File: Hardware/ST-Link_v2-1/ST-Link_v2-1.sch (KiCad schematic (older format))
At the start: 40 parts, among them J1 Conn_01x06, J2 USB_C_Receptacle, U1 STM32F103CBTx, U2 LP5907MFX-3.3, Y1 8Mhz

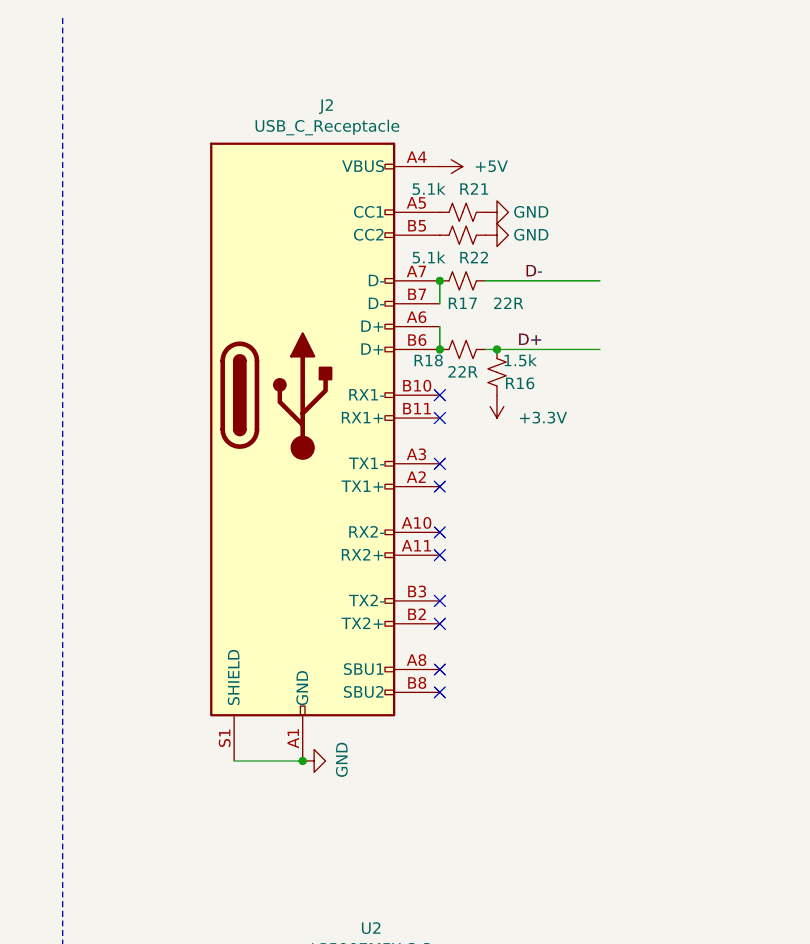
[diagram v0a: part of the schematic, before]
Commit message: V2.1 11/12/2021
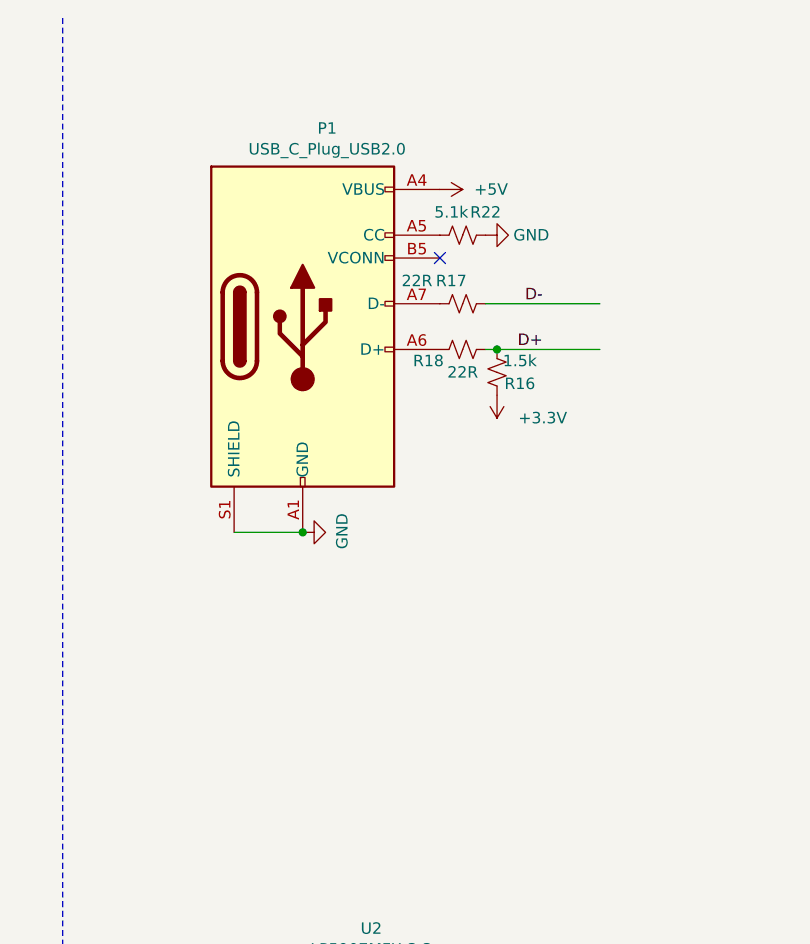
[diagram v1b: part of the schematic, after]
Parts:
- removed J2: USB_C_Receptacle, HKUST_RT_CONN:USB_C_MALE, symbol HKUST_RT_CONN:USB_C_Receptacle
- removed R21: 5.1k, HKUST_RT_RCL:R_0805_2012Metric, symbol HKUST_RT_RCL:R_Small_US
- added P1: USB_C_Plug_USB2.0, HKUST_RT_CONN:USB_C_MALE, symbol HKUST_RT_CONN:USB_C_Plug_USB2.0
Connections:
- wire segments 72 -> 70
- no-connect marks 28 -> 19
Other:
- moved on the sheet: R17
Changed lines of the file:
@@
 L HKUST_RT_RCL:R_Small_US R17
 U 1 1 619A5D6F
-P 6350 1650
-F 0 "R17" V 6450 1650 50  0000 C CNN
-F 1 "22R" V 6450 1850 50  0000 C CNN
-F 2 "HKUST_RT_RCL:R_0805_2012Metric" H 6418 1559 50  0001 L CNN
-F 3 "" H 6350 1650 50  0001 C CNN
-	1    6350 1650
+P 6350 1750
+F 0 "R17" V 6250 1700 50  0000 C CNN
+F 1 "22R" V 6250 1550 50  0000 C CNN
+F 2 "HKUST_RT_RCL:R_0805_2012Metric" H 6418 1659 50  0001 L CNN
+F 3 "" H 6350 1750 50  0001 C CNN
+	1    6350 1750
 	0    1    1    0
 $EndComp
@@
 Wire Notes Line style solid rgb(0, 0, 0)
 	4600 500  4600 7750
-Text Label 6700 1650 2    50   ~ 0
+Text Label 6700 1750 2    50   ~ 0
 D-
 Text Label 6700 1950 2    50   ~ 0
@@
 $EndComp
 $Comp
-L power:GND #PWR0102
-U 1 1 619EB02D
-P 5650 3750
-F 0 "#PWR0102" H 5650 3500 50  0001 C CNN
-F 1 "GND" H 5655 3577 50  0000 C CNN
-F 2 "" H 5650 3750 50  0001 C CNN
-F 3 "" H 5650 3750 50  0001 C CNN
-	1    5650 3750
-	0    -1   -1   0
-$EndComp
-$Comp
-L power:+5V #PWR0103
-U 1 1 619F8999
-P 6250 1150
-F 0 "#PWR0103" H 6250 1000 50  0001 C CNN
-F 1 "+5V" V 6250 1300 50  0000 L CNN
-F 2 "" H 6250 1150 50  0001 C CNN
-F 3 "" H 6250 1150 50  0001 C CNN
-	1    6250 1150
-	0    1    1    0
-$EndComp
-$Comp
-L HKUST_RT_RCL:R_Small_US R21
-U 1 1 61A837A5
-P 6350 1350
-F 0 "R21" V 6450 1300 50  0000 C CNN
-F 1 "5.1k" V 6450 1500 50  0000 C CNN
-F 2 "HKUST_RT_RCL:R_0805_2012Metric" H 6418 1259 50  0001 L CNN
-F 3 "" H 6350 1350 50  0001 C CNN
-	1    6350 1350
-	0    -1   -1   0
-$EndComp
-$Comp
 L power:GND #PWR0104
 U 1 1 61AA0D72
@@
 $EndComp
 Wire Wire Line
-	6950 1650 6450 1650
+	6950 1750 6450 1750
 $Comp
 L HKUST_RT_RCL:Crystal_GND24_Small Y1
@@
 	-1   0    0    1
 $EndComp
-Wire Wire Line
-	5350 3750 5650 3750
-NoConn ~ 6250 3050
-NoConn ~ 6250 2750
-NoConn ~ 6250 2850
-NoConn ~ 6250 3350
-NoConn ~ 6250 3450
-NoConn ~ 6250 2450
-NoConn ~ 6250 2550
-NoConn ~ 6250 2150
-Connection ~ 5650 3750
-$Comp
-L HKUST_RT_CONN:USB_C_Receptacle J2
-U 1 1 61AC3D44
-P 5650 2150
-F 0 "J2" H 5757 3417 50  0000 C CNN
-F 1 "USB_C_Receptacle" H 5757 3326 50  0000 C CNN
-F 2 "HKUST_RT_CONN:USB_C_MALE" H 5800 2150 50  0001 C CNN
-F 3 "https://www.usb.org/sites/default/files/documents/usb_type-c.zip" H 5800 2150 50  0001 C CNN
-	1    5650 2150
-	1    0    0    -1
-$EndComp
-NoConn ~ 6250 2250
-Wire Wire Line
-	6250 1650 6250 1750
-Wire Wire Line
-	6250 1850 6250 1950
+NoConn ~ 6250 1550
 $Comp
 L HKUST_RT_RCL:R_Small_US R22
 U 1 1 61AF811F
 P 6350 1450
-F 0 "R22" V 6250 1400 50  0000 C CNN
-F 1 "5.1k" V 6250 1600 50  0000 C CNN
+F 0 "R22" V 6450 1350 50  0000 C CNN
+F 1 "5.1k" V 6450 1500 50  0000 C CNN
 F 2 "HKUST_RT_RCL:R_0805_2012Metric" H 6418 1359 50  0001 L CNN
 F 3 "" H 6350 1450 50  0001 C CNN
@@
 	0    -1   -1   0
 $EndComp
-$Comp
-L power:GND #PWR0105
-U 1 1 61AFA16E
-P 6450 1350
-F 0 "#PWR0105" H 6450 1100 50  0001 C CNN
-F 1 "GND" V 6450 1150 50  0000 C CNN
-F 2 "" H 6450 1350 50  0001 C CNN
-F 3 "" H 6450 1350 50  0001 C CNN
-	1    6450 1350
-	0    -1   -1   0
-$EndComp
-Connection ~ 6250 1650
-Connection ~ 6250 1950
-NoConn ~ 6250 3150
 Wire Wire Line
 	2900 1550 2800 1550
@@
 	0    1    1    0
 $EndComp
+$Comp
+L power:+5V #PWR0103
+U 1 1 619F8999
+P 6250 1250
+F 0 "#PWR0103" H 6250 1100 50  0001 C CNN
+F 1 "+5V" V 6250 1400 50  0000 L CNN
+F 2 "" H 6250 1250 50  0001 C CNN
+F 3 "" H 6250 1250 50  0001 C CNN
+	1    6250 1250
+	0    1    1    0
+$EndComp
+$Comp
+L HKUST_RT_CONN:USB_C_Plug_USB2.0 P1
+U 1 1 61B83845
+P 5650 1850
+F 0 "P1" H 5757 2717 50  0000 C CNN
+F 1 "USB_C_Plug_USB2.0" H 5757 2626 50  0000 C CNN
+F 2 "HKUST_RT_CONN:USB_C_MALE" H 5800 1850 50  0001 C CNN
+F 3 "https://www.usb.org/sites/default/files/documents/usb_type-c.zip" H 5800 1850 50  0001 C CNN
+	1    5650 1850
+	1    0    0    -1
+$EndComp
+$Comp
+L power:GND #PWR0102
+U 1 1 619EB02D
+P 5650 2750
+F 0 "#PWR0102" H 5650 2500 50  0001 C CNN
+F 1 "GND" H 5655 2577 50  0000 C CNN
+F 2 "" H 5650 2750 50  0001 C CNN
+F 3 "" H 5650 2750 50  0001 C CNN
+	1    5650 2750
+	0    -1   -1   0
+$EndComp
+Wire Wire Line
+	5350 2750 5650 2750
+Connection ~ 5650 2750
 $EndSCHEMATC
